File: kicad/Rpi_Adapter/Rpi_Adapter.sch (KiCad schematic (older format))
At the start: 3 parts, among them P1 CONN_02X20, P2 CONN_02X03

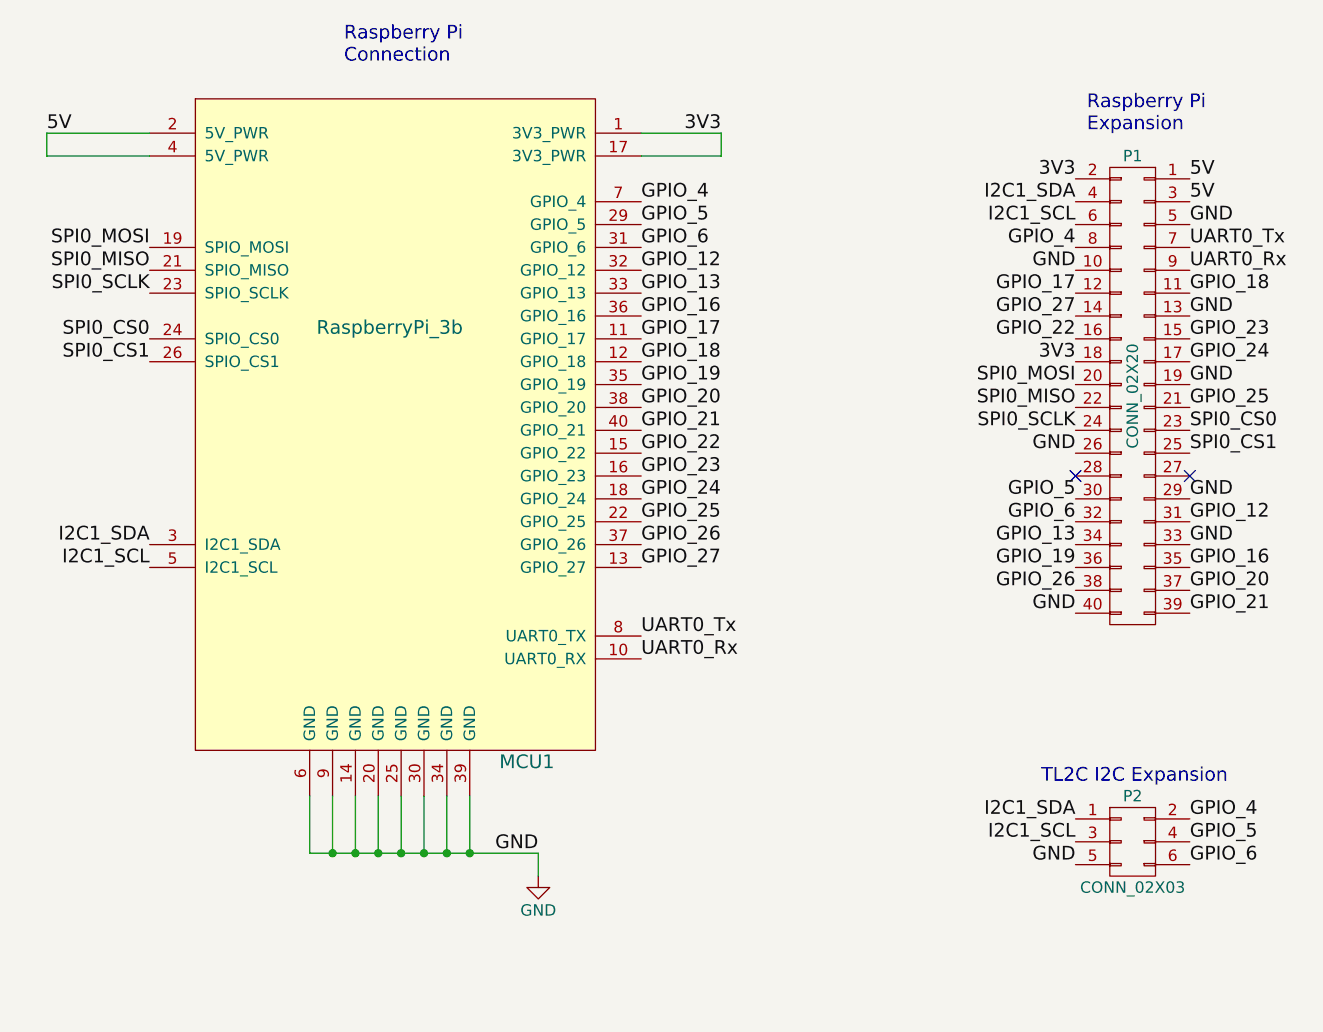
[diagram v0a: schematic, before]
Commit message: Created the layout and submitted to OSH Park
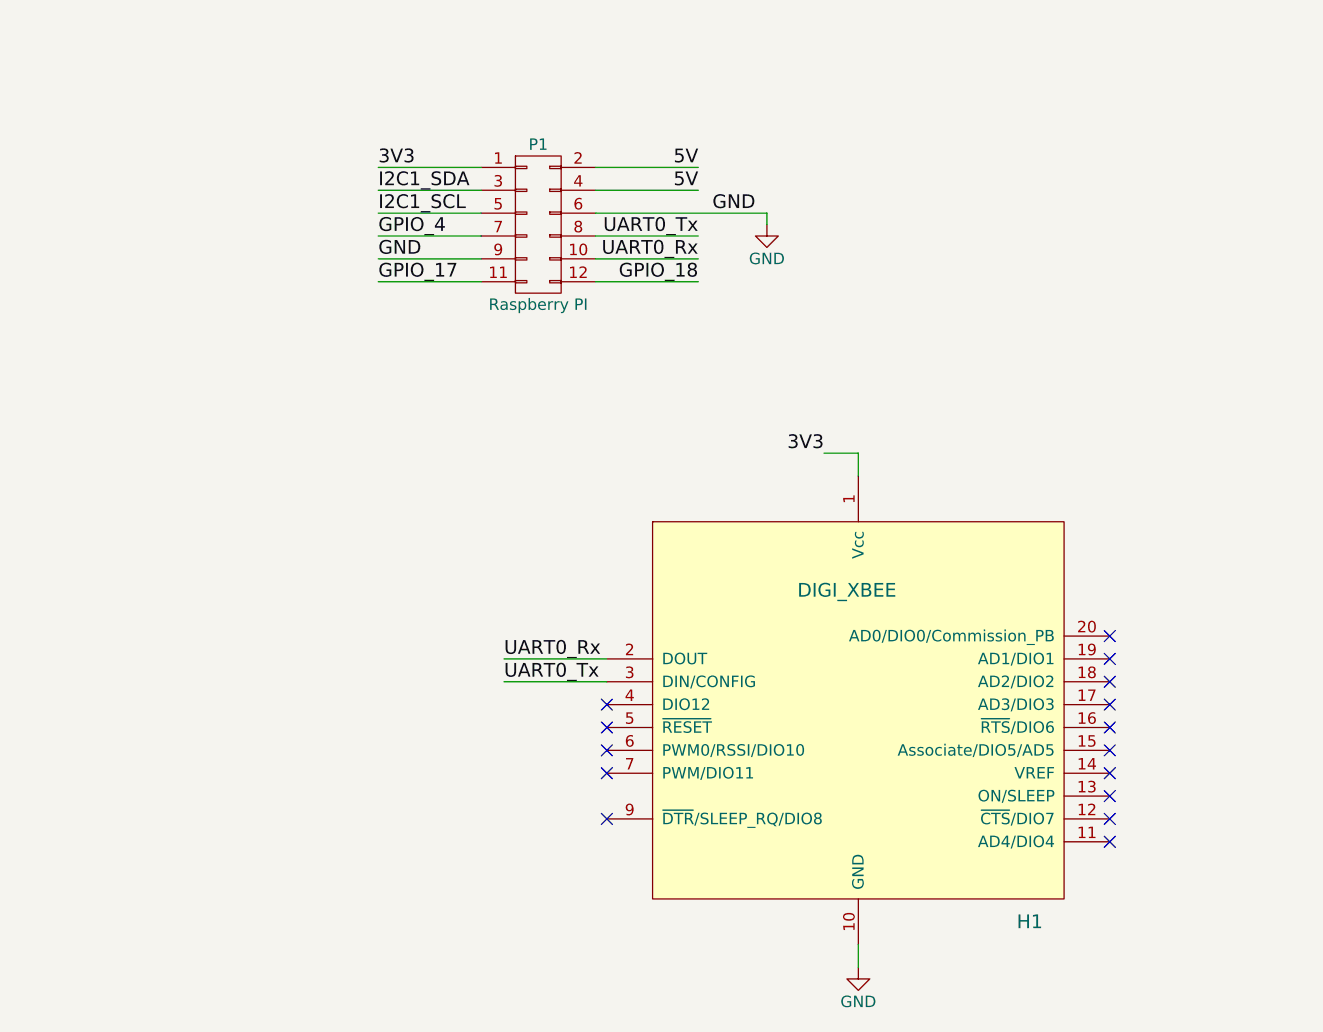
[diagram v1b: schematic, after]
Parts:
- removed MCU1: RaspberryPi_3b, Socket_Strips:Socket_Strip_Straight_2x10_Pitch2.54mm_SMD, symbol RaspberryPi_3b
- removed P1: CONN_02X20, Pin_Headers:Pin_Header_Straight_2x20_Pitch2.54mm, symbol CONN_02X20
- removed P2: CONN_02X03, Pin_Headers:Pin_Header_Straight_2x03_Pitch2.54mm, symbol CONN_02X03
- added H1: DIGI_XBEE, Rpi_Adapter_Footprints:XBEE_S2C_Short, symbol DIGI_XBEE
- added P1: Raspberry PI, Socket_Strips:Socket_Strip_Straight_2x06_Pitch2.54mm, symbol CONN_02X06
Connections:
- net 3V3: now also H1.1 (Vcc), P1.1 (P1)
- net 5V: now also P1.2 (P2), P1.4 (P4)
- net GND: now also H1.10 (GND), P1.6 (P6), P1.9 (P9)
- net GPIO_17: now also P1.11 (P11)
- net GPIO_18: now also P1.12 (P12)
- net GPIO_4: now also P1.7 (P7)
- net I2C1_SCL: now also P1.5 (P5)
- net I2C1_SDA: now also P1.3 (P3)
- net UART0_Rx: now also H1.2 (DOUT), P1.10 (P10)
- net UART0_Tx: now also H1.3 (DIN/CONFIG), P1.8 (P8)
- no-connect marks 2 -> 15
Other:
- note removed: "Raspberry Pi\nConnection"
- note removed: "Raspberry Pi\nExpansion"
- note removed: "TL2C I2C Expansion"
